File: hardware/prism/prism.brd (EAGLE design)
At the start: 100 x 79 mm, 174 parts, among them IC1 XMEGA128-A1, IC2 74LVC4245APW, IC3 LM2731XMF, IC4 74LVC4245APW, IC5 LM25011MY, IC6 NCV78M05BDTRKG, IC7 NRF24L01+, IC8 MAX3232CSE, T1 MMBT2222LT1G, T2 NTGS4111PT1G, T3 MMBT2222LT1G, T4 MMBT2222LT1G, T5 NTGS4111PT1G, T6 MMBT2222LT1G, T7 MMBT2222LT1G, T8 NTGS4111PT1G

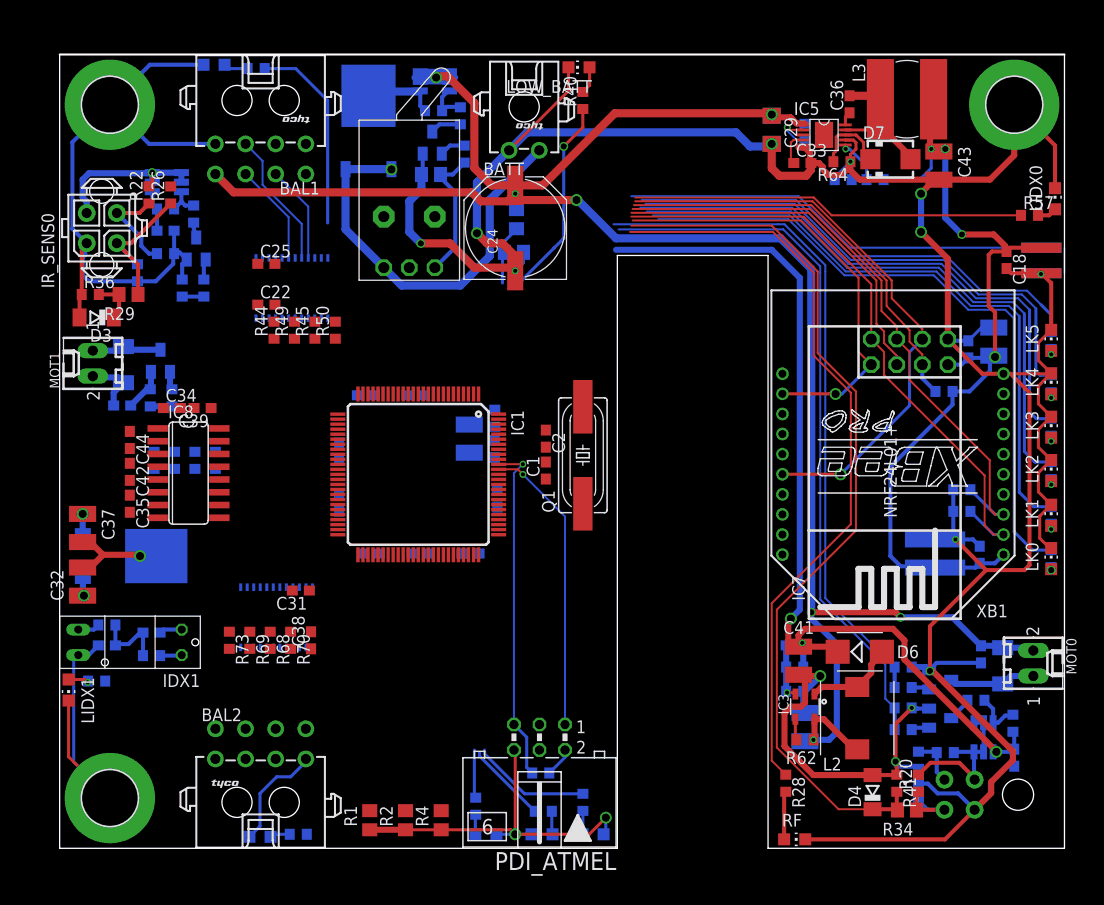
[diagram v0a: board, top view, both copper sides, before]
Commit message: bord routed, ready to review
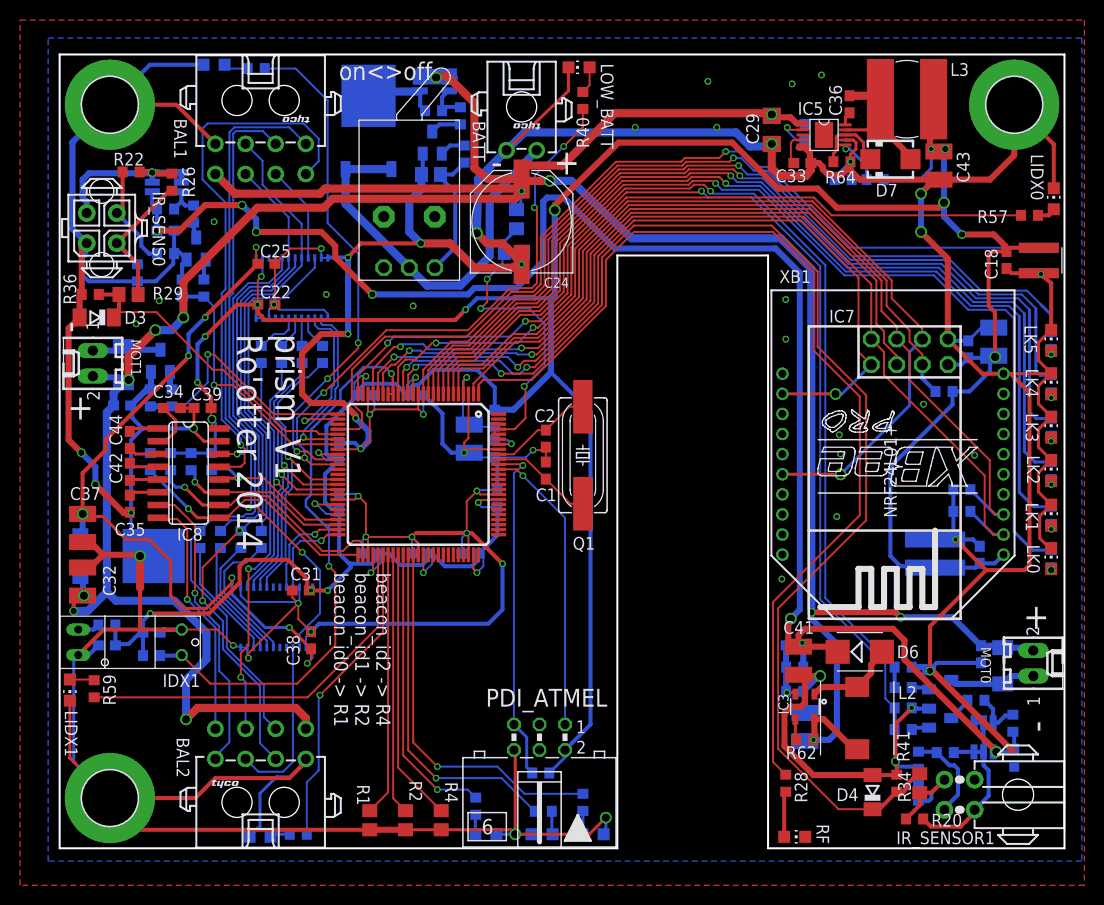
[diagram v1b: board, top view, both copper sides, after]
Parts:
- moved R70 13.5 mm to (14.0, 30.7), flipped to the bottom, turned to 90 degrees
- moved R68 11.2 mm to (16.0, 30.7), flipped to the bottom, turned to 90 degrees
- moved R73 10.5 mm to (20.1, 30.7), flipped to the bottom, turned to 90 degrees
- moved R69 10.1 mm to (18.0, 30.7), flipped to the bottom, turned to 90 degrees
- moved R37 6.48 mm to (9.02, 38.5)
- moved R30 3.69 mm to (15.1, 38.5)
- moved R33 3.69 mm to (13.1, 38.5)
- moved R20 3.58 mm to (85.1, 2.92), turned to 0 degrees
- moved R34 2.95 mm to (85.6, 6.48), turned to 90 degrees
- moved R22 2.90 mm to (7.11, 67.3), turned to 0 degrees
- moved R44 2.73 mm to (20.1, 49.1), flipped to the bottom
- moved R45 2.73 mm to (24.1, 49.1), flipped to the bottom
- moved R49 2.73 mm to (22.1, 49.1), flipped to the bottom
- moved R50 2.73 mm to (26.2, 49.1), flipped to the bottom
- moved R39 2.42 mm to (11.0, 38.5)
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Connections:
- removed net LED_EAST: IC1.56
- removed net LED_NORTH: IC1.62
- removed net LED_WEST: IC1.95
- removed net N$32: IC1.68, R40.1
- removed net N$36: IC1.66, R32.2
- new net LOW_BAT_LED_3V3: IC1.36, R40.1
- new net SYNC1_LED_3V3: IC1.35, R32.2
- net BEACON_ID_0_3V3: now also IC1.57; no longer IC1.5
- net BEACON_ID_1_3V3: now also IC1.58; no longer IC1.6
- net BEACON_ID_2_3V3: now also IC1.59; no longer IC1.7
- net INT0_0_3V3: now also IC1.39, IC4.17; no longer IC4.16
- net INT0_1_3V3: now also IC1.40, IC4.16; no longer IC4.17
- net INT1_0_3V3: now also IC1.41, IC4.15; no longer IC4.18
- net INT1_1_3V3: now also IC1.42, IC4.14; no longer IC4.19
- net IR_SENSOR_0_OUTPUT_3V3: now also IC1.30; no longer IC1.17
- net IR_SENSOR_1_OUTPUT_3V3: now also IC1.15; no longer IC1.37
- net LED_INDEX_0_3V3: now also IC1.6; no longer IC1.81
- net LED_INDEX_1_3V3: now also IC1.55; no longer IC1.82
- net LK0_3V3: now also IC1.7; no longer IC1.75
- net LK1_3V3: now also IC1.8; no longer IC1.76
- net LK2_3V3: now also IC1.9; no longer IC1.77
- net LK3_3V3: now also IC1.10; no longer IC1.78
- net LK4_3V3: now also IC1.11; no longer IC1.79
- net LK5_3V3: now also IC1.12; no longer IC1.80
- net MIRROR_INDEX_0_3V3: now also IC1.29; no longer IC1.18
- net MIRROR_INDEX_1_3V3: now also IC1.18, IC1.19; no longer IC1.38
- net N$10: now also IC1.60; no longer IC1.71
- net N$12: now also IC1.62; no longer IC1.72
- net N$23: now also SW_BATT.2; no longer SW_BATT.1
- net N$28: now also IC1.1; no longer IC1.65
- net N$31: now also IC1.56; no longer IC1.67
- net N$47: now also IC4.10; no longer IC4.5
- net N$53: now also IC4.9; no longer IC4.6
- net N$54: now also IC4.7; no longer IC4.8
- net N$55: now also IC4.8; no longer IC4.7
- net N$9: now also IC1.61; no longer IC1.70
- net NRF_CSN_3V3: now also IC1.2; no longer IC1.35
- net NRF_MOSI_3V3: now also IC1.20; no longer IC1.30
- net ON/OFF_SENSOR_0_3V3: now also IC1.32; no longer IC1.27
- net ON/OFF_SENSOR_1_3V3: now also IC1.17; no longer IC1.28
- net RX_0_3V3: now also IC1.47, R30.2; no longer IC1.51, R37.1
- net RX_1_3V3: now also IC1.51, R37.1; no longer IC1.47, R30.2
- net SYNC_IN_0_3V3: now also IC1.27; no longer IC1.19
- net SYNC_IN_1_3V3: now also IC1.31; no longer IC1.20
- net SYNC_OUT_0_3V3: now also IC1.50, IC4.21; no longer IC1.21, IC4.15
- net SYNC_OUT_0_5V: now also IC4.3; no longer IC4.9
- net SYNC_OUT_1_3V3: now also IC1.49, IC4.20; no longer IC1.22, IC4.14
- net SYNC_OUT_1_5V: now also IC4.4; no longer IC4.10
- net TX_0_3V3: now also IC1.48, R33.2; no longer IC1.52, R39.1
- net TX_1_3V3: now also IC1.52, R39.1; no longer IC1.48, R33.2
- net XBEE_CTS_3V3/NRF_IRQ_3V3: now also IC1.16; no longer IC1.57
- net XBEE_RTS_3V3/NRF_CE_3V3: now also IC1.5; no longer IC1.58
- net XBEE_RX_3V3/NRF_MISO_3V3: now also IC1.21; no longer IC1.31
- net XBEE_TX_3V3/NRF_SCK_3V3: now also IC1.22; no longer IC1.32
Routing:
- net +3V3: track 94.9 -> 398.7 mm, vias 4 -> 23
- net GND: track 520.7 -> 811.7 mm, vias 16 -> 57
- net VBAT: track 223.9 -> 338.3 mm, vias 8 -> 13
- net +5V: track 2.94 -> 75.5 mm, vias 1 -> 7
- net +15V: track 99.9 -> 161.7 mm, vias 3 -> 7
- net SYNC_OUT_0_5V: track 0.00 -> 61.5 mm, vias 0 -> 2
- net INT0_1_5V: track 0.00 -> 60.1 mm, vias 0 -> 2
- net INT1_1_5V: track 0.00 -> 59.1 mm
- net LOW_BAT_LED_3V3: track 0.00 -> 56.7 mm, vias 0 -> 4
- net MIRROR_INDEX_1_3V3: track 2.18 -> 57.5 mm, vias 0 -> 2
- net RX_0_RS232: track 0.00 -> 54.4 mm, vias 0 -> 1
- net SYNC_IN_1_5V: track 0.00 -> 54.1 mm, vias 0 -> 2
- net SYNC1_LED_3V3: track 0.00 -> 51.0 mm, vias 0 -> 3
- net MIRROR_INDEX_0_3V3: track 42.9 -> 92.6 mm, vias 0 -> 1
- net TX_0_RS232: track 0.00 -> 44.1 mm, vias 0 -> 1
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- added copper zone on layer 1, net GND
- added copper zone on layer 16, net GND
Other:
- board text added: "+"
- board text added: "-"
- board text added: "beacon_id2 -> R4 beacon_id1 -> R2 beacon_id0 -> R1"
- board text added: "on<>off"
- board text added: "prism_V1 Ro'otter 2014"
